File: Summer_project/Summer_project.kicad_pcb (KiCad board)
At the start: 2 copper layers, 98.4 x 83.5 mm, 16 parts, among them Q3 2N3904, Q4 2N3904, SW1 SW_Push

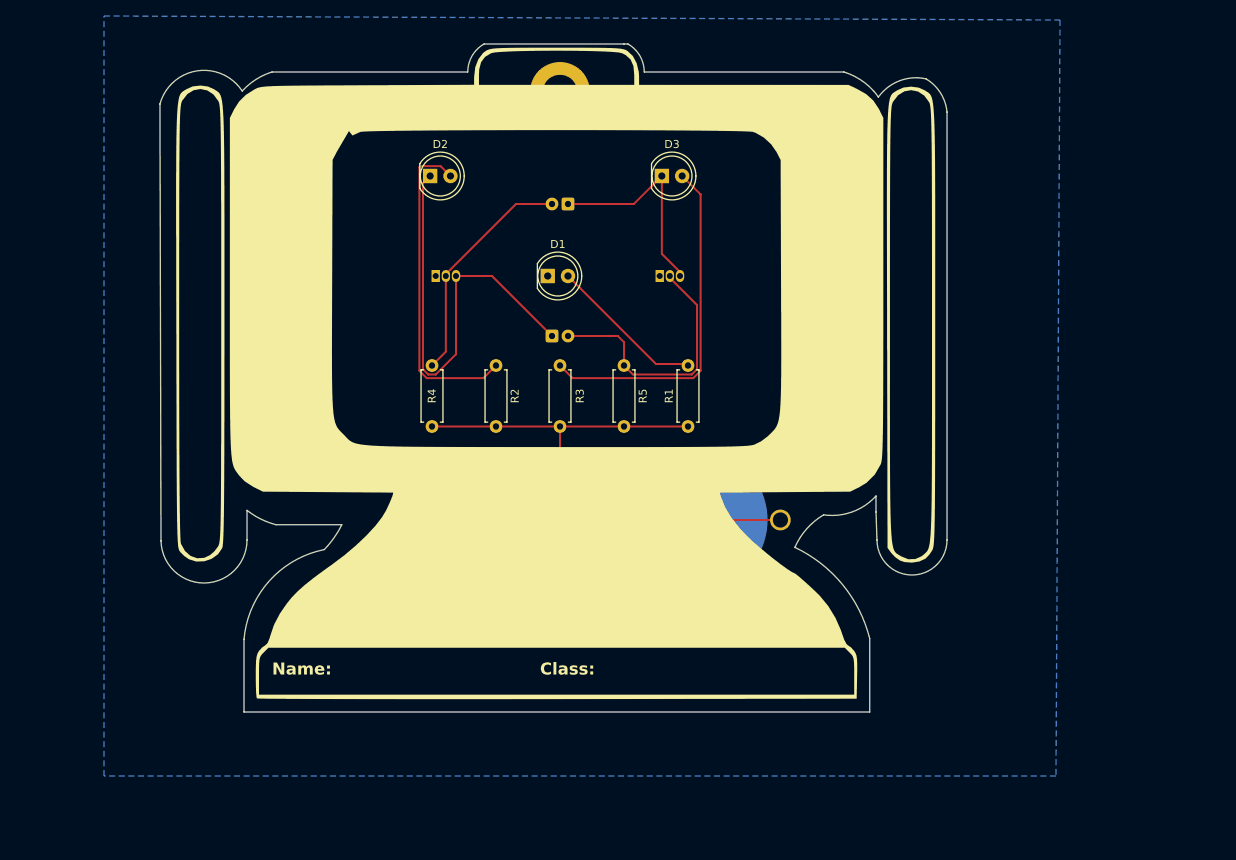
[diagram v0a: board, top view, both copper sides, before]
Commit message: Name_without_silicon_hole_6mm
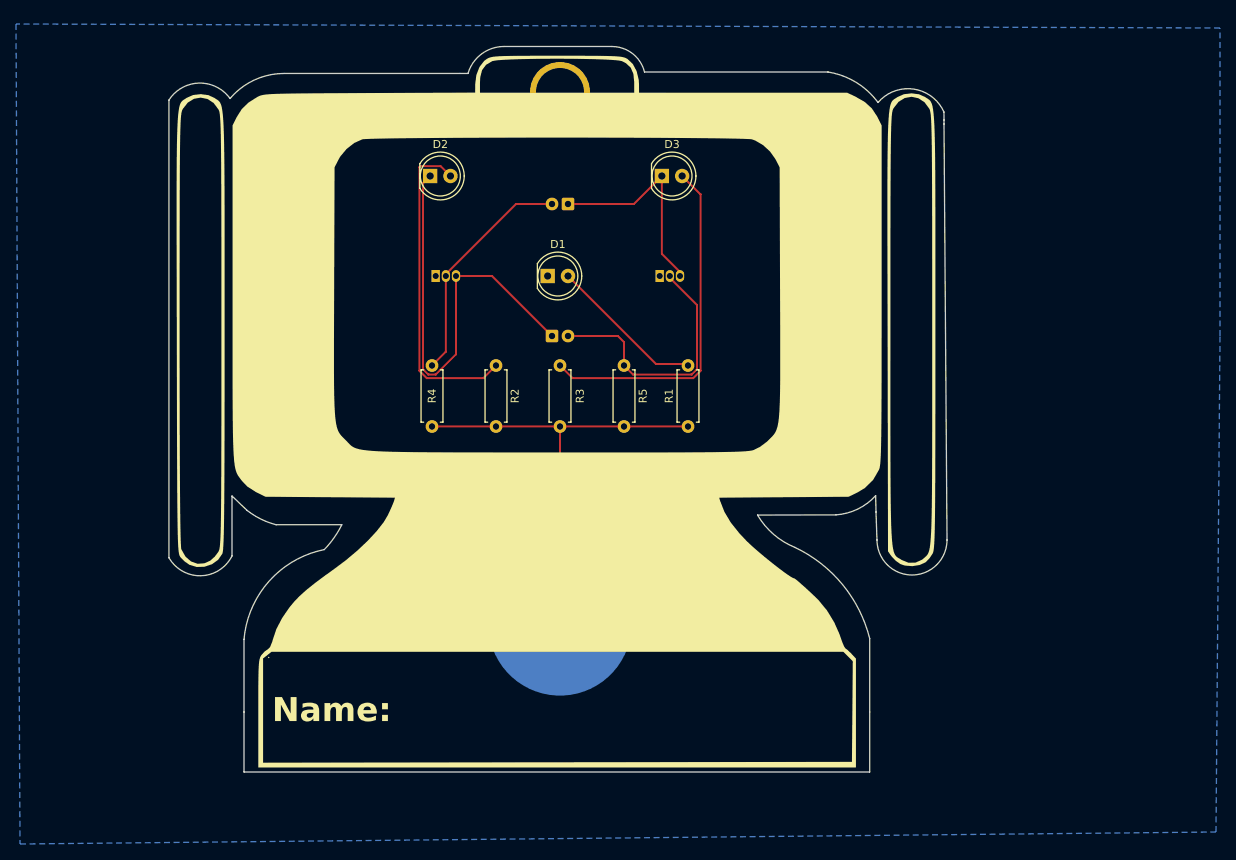
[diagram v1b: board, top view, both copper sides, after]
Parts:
- removed the G*** at (149.0, 125.0)
- added G***: LOGO, Summer_project:RSC_robot_with_name, F.Cu at (149.3, 133.3)
- added G***: LOGO, Summer_project:RSC_qr_code, B.Cu at (226.0, 40.9)
- moved BT1 21.4 mm to (149.5, 115.5)
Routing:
- net Net-(BT1-+): track 31.3 -> 39.4 mm
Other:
- board size 98.4 x 83.5 mm -> 97.3 x 90.7 mm
- board text added: "Designed by: Timur Kedrov"
- board text added: "RSC Summer School Badge"
- board text added: "Rev 1.0 2026"
- board text removed: "Class:"
